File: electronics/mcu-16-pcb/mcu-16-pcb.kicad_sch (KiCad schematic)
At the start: 32 parts, among them J1 HRO_TYPE-C-31-M-12, J2 FFC Connector, U1 AP2112K-3.3, U2 W25Q64JVXGIQ, U3 Raspberry_Pi_RP2040, Y1 12MHz

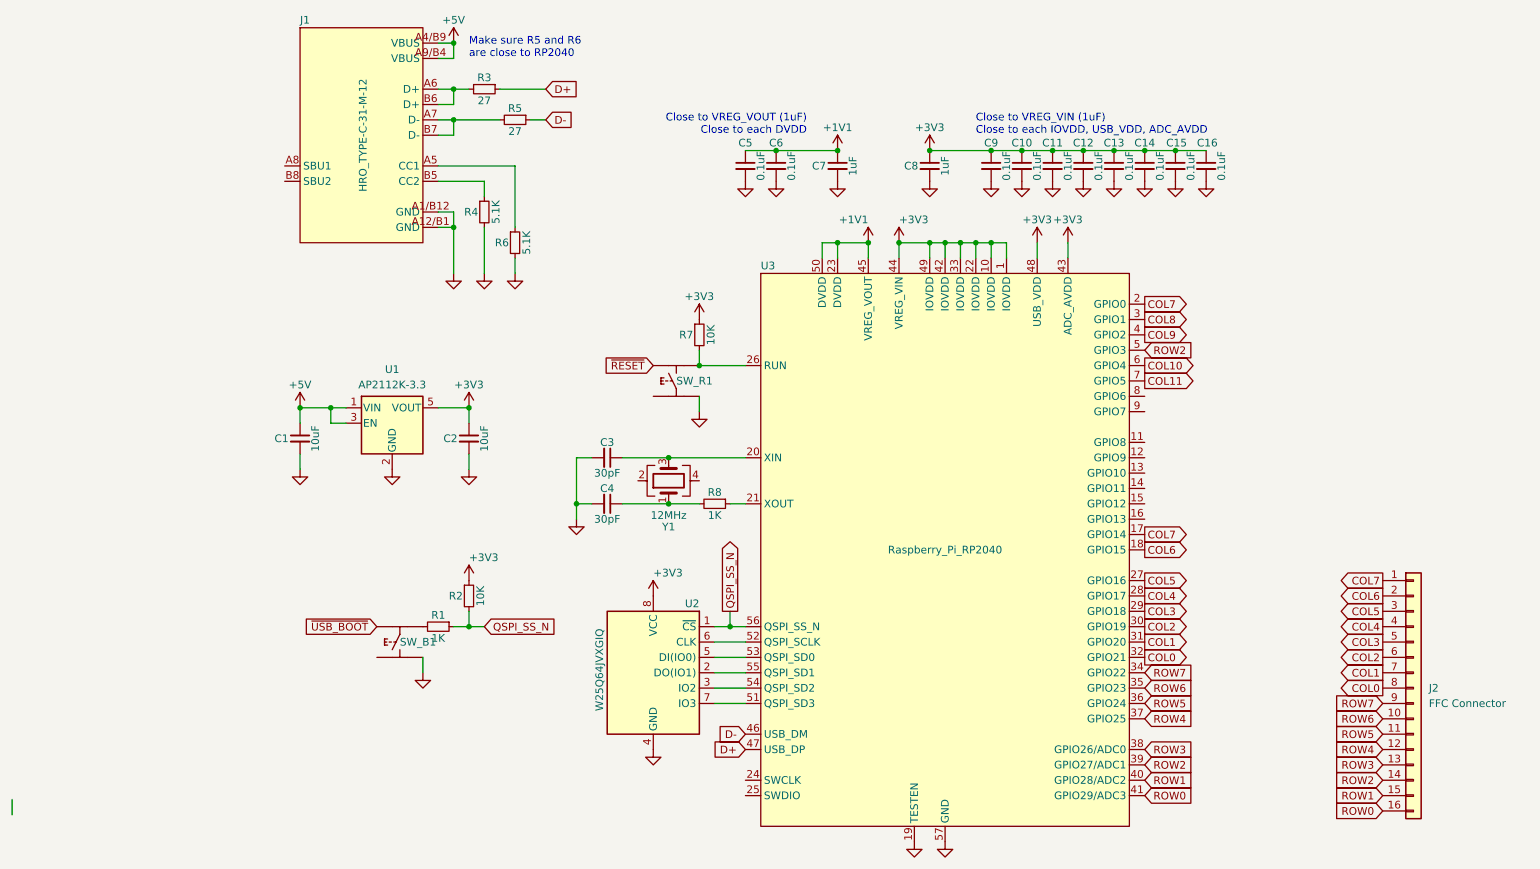
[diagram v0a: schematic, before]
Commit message: WIP Update
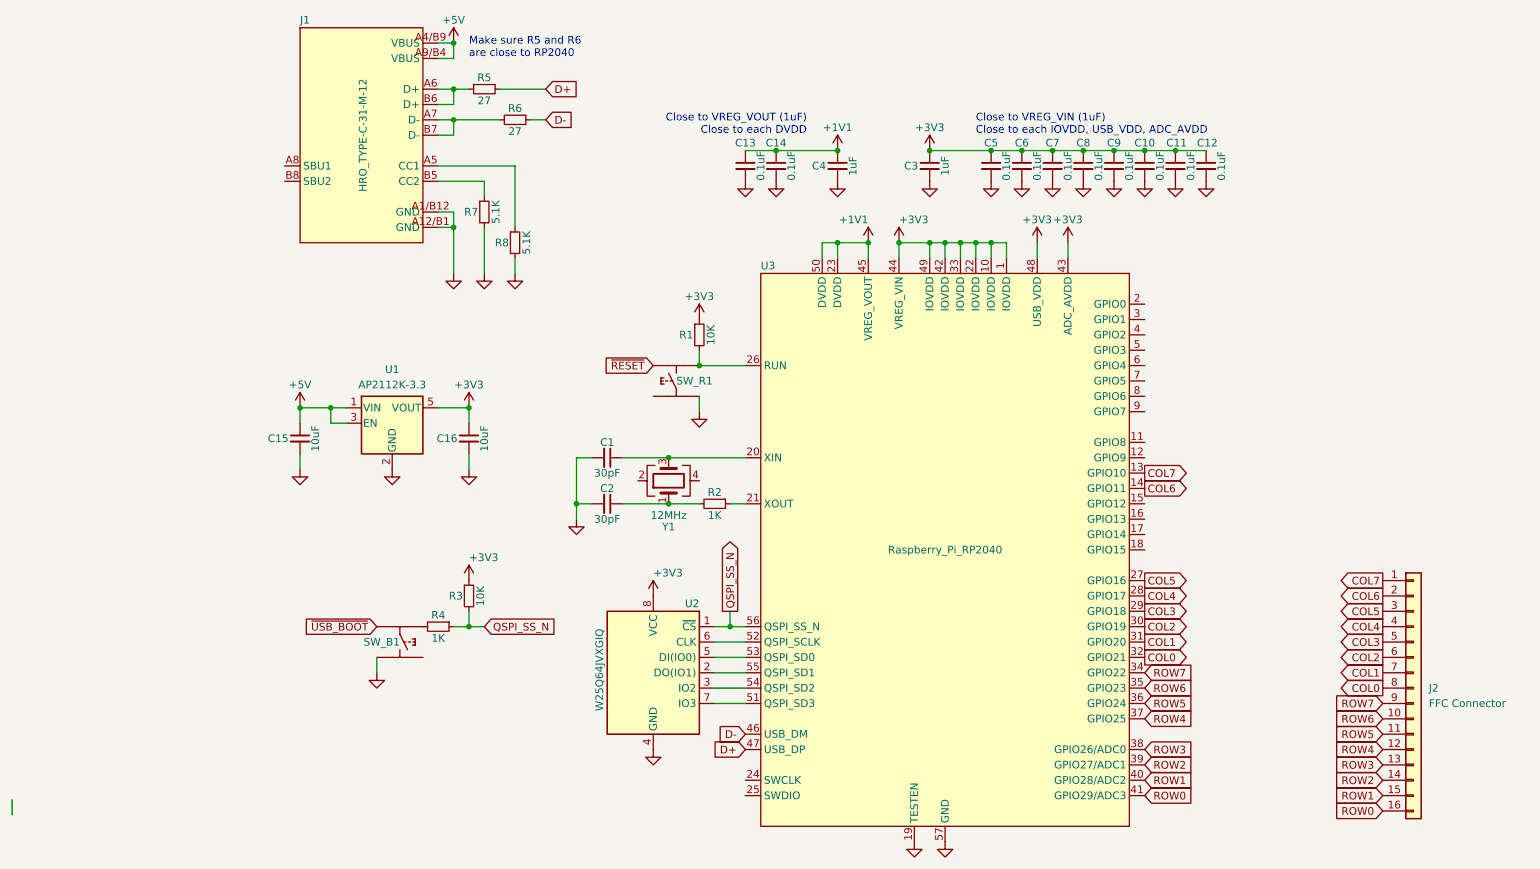
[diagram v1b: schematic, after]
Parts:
- renumbered C3 to C1, C14 to C10, C15 to C11, C16 to C12, C5 to C13, C6 to C14, C1 to C15, C2 to C16, C4 to C2, C8 to C3, C7 to C4, C9 to C5, C10 to C6, C11 to C7, C12 to C8, C13 to C9, R7 to R1, R8 to R2, R2 to R3, R1 to R4, R3 to R5, R5 to R6, R4 to R7, R6 to R8
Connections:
- net COL6: now also U3.14 (GPIO11); no longer U3.18 (GPIO15)
- net COL7: now also U3.13 (GPIO10); no longer U3.17 (GPIO14), U3.2 (GPIO0)
- net ROW2: no longer U3.5 (GPIO3)
- net ~{USB_BOOT}: now also SW_B1.1; no longer SW_B1.2
- net at R4.2: now also SW_B1.2; no longer SW_B1.1
- net COL10: no longer names the net of U3.6 (GPIO4)
- net COL11: no longer names the net of U3.7 (GPIO5)
- net COL8: no longer names the net of U3.3 (GPIO1)
- net COL9: no longer names the net of U3.4 (GPIO2)

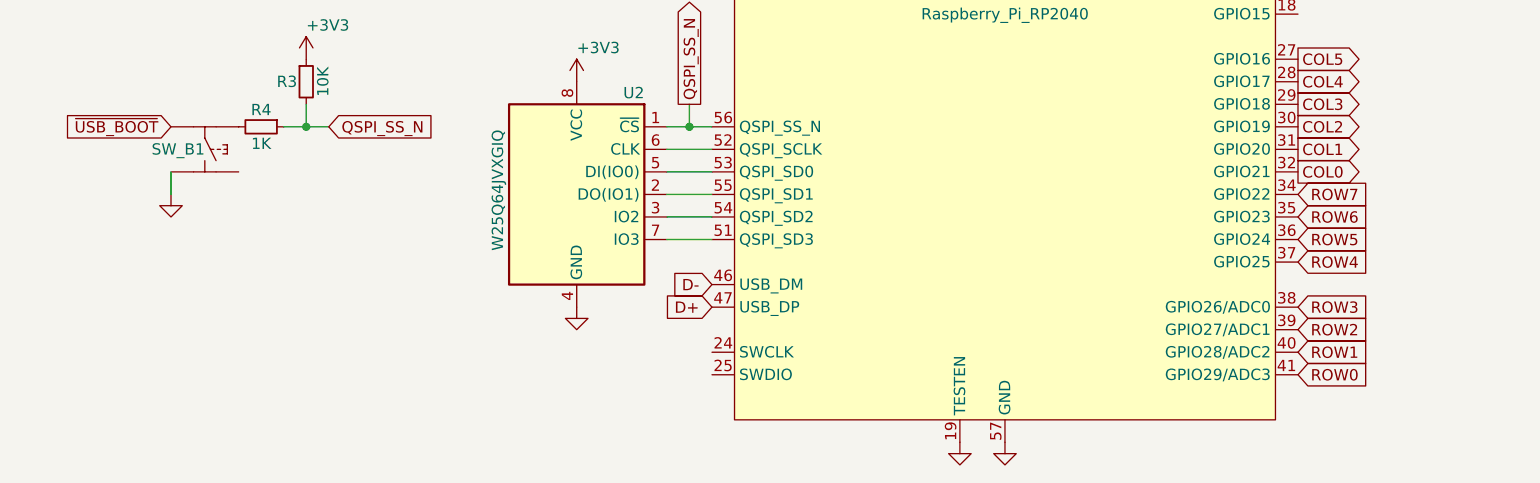
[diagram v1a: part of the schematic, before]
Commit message: Update MCU 16 pcb
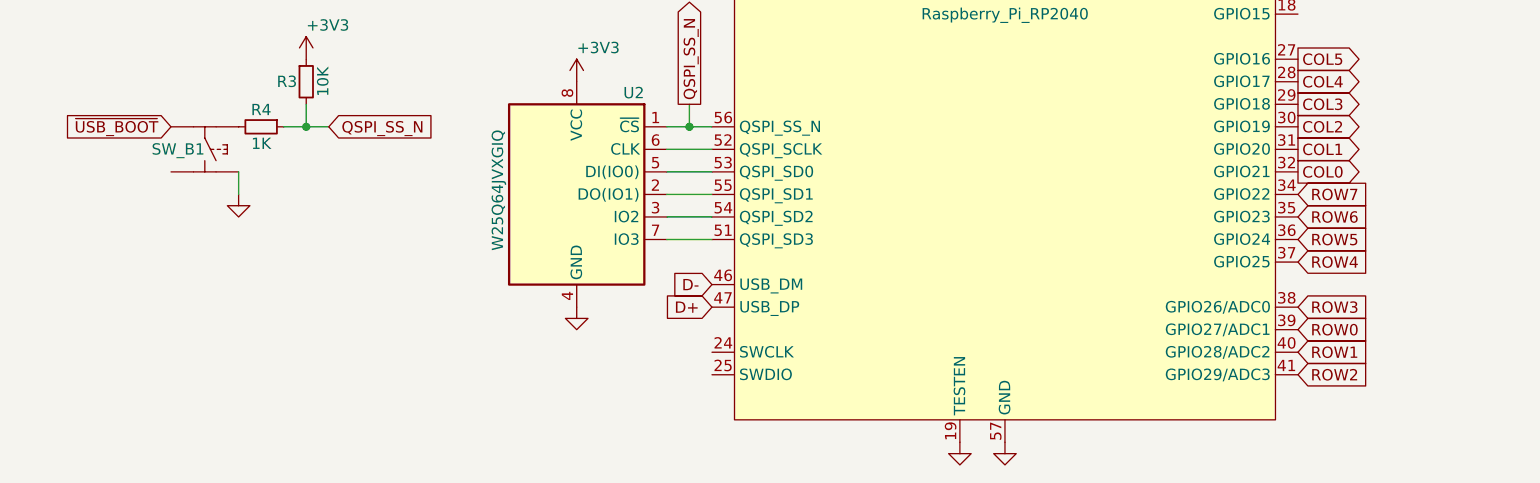
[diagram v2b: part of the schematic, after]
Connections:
- net GND: now also SW_B1.4; no longer SW_B1.3
- net ROW0: now also U3.39 (GPIO27/ADC1); no longer U3.41 (GPIO29/ADC3)
- net ROW2: now also U3.41 (GPIO29/ADC3); no longer U3.39 (GPIO27/ADC1)
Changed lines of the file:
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@@
 	(wire
 		(pts
-			(xy 35.56 127) (xy 35.56 129.54)
+			(xy 43.18 127) (xy 43.18 129.54)
 		)
 		(stroke
@@
 	(global_label "ROW2"
 		(shape input)
-		(at 162.56 144.78 0)
+		(at 162.56 149.86 0)
 		(fields_autoplaced yes)
 		(effects
@@
 		)
 		(property "Intersheetrefs" "${INTERSHEET_REFS}"
-			(at 170.8066 144.78 0)
+			(at 170.8066 149.86 0)
 			(effects
 				(font
@@
 	(global_label "ROW0"
 		(shape input)
-		(at 162.56 149.86 0)
+		(at 162.56 144.78 0)
 		(fields_autoplaced yes)
 		(effects
@@
 		)
 		(property "Intersheetrefs" "${INTERSHEET_REFS}"
-			(at 170.8066 149.86 0)
+			(at 170.8066 144.78 0)
 			(effects
 				(font
@@
 	(symbol
 		(lib_id "power:GND")
-		(at 35.56 129.54 0)
+		(at 43.18 129.54 0)
 		(unit 1)
 		(exclude_from_sim no)
@@
 		(fields_autoplaced yes)
 		(property "Reference" "#PWR04"
-			(at 35.56 135.89 0)
+			(at 43.18 135.89 0)
 			(effects
 				(font
@@
 		)
 		(property "Value" "GND"
-			(at 35.56 134.62 0)
+			(at 43.18 134.62 0)
 			(effects
 				(font
@@
 		)
 		(property "Footprint" ""
-			(at 35.56 129.54 0)
+			(at 43.18 129.54 0)
 			(effects
 				(font
@@
 		)
 		(property "Datasheet" ""
-			(at 35.56 129.54 0)
+			(at 43.18 129.54 0)
 			(effects
 				(font
@@
 		)
 		(property "Description" ""
-			(at 35.56 129.54 0)
-			(effects
-				(font
+			(at 43.18 129.54 0)
+			(effects
+				(font

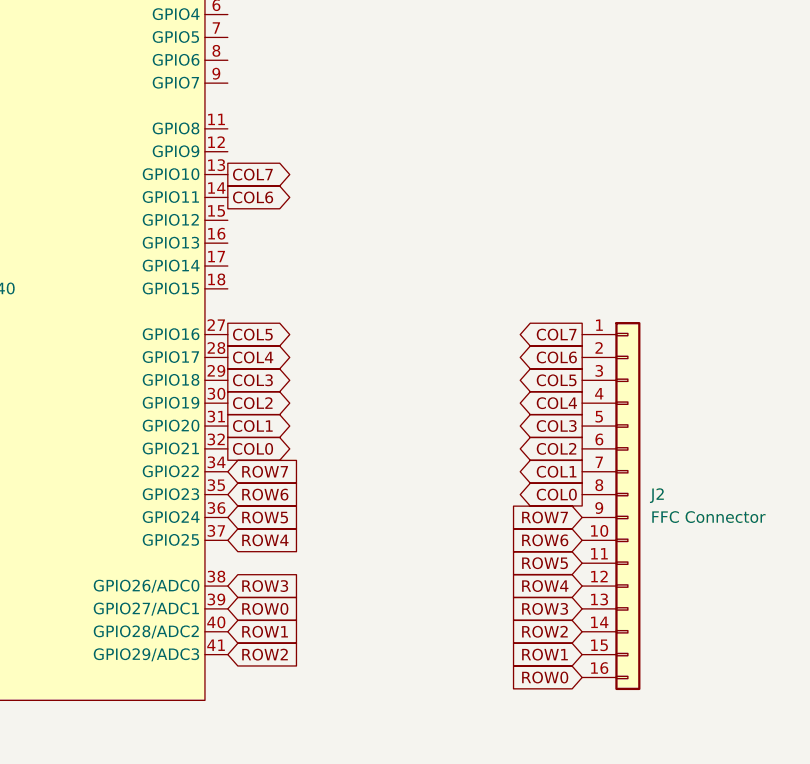
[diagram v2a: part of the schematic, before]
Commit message: Update MCU 16 pcb
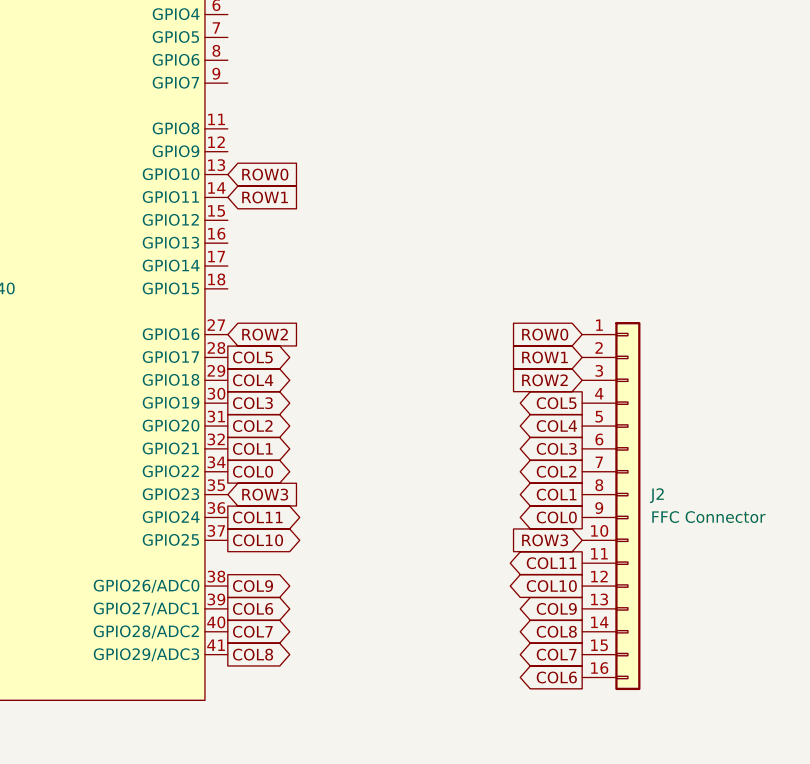
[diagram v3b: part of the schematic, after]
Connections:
- net ROW6 is gone; now on net ROW3: J2.10 (Pin_10), U3.35 (GPIO23)
- net ROW7 is gone; now on net COL0: J2.9 (Pin_9), U3.34 (GPIO22)
- net COL0: no longer J2.8 (Pin_8), U3.32 (GPIO21)
- net COL1: now also J2.8 (Pin_8), U3.32 (GPIO21); no longer J2.7 (Pin_7), U3.31 (GPIO20)
- net COL2: now also J2.7 (Pin_7), U3.31 (GPIO20); no longer J2.6 (Pin_6), U3.30 (GPIO19)
- net COL3: now also J2.6 (Pin_6), U3.30 (GPIO19); no longer J2.5 (Pin_5), U3.29 (GPIO18)
- net COL4: now also J2.5 (Pin_5), U3.29 (GPIO18); no longer J2.4 (Pin_4), U3.28 (GPIO17)
- net COL5: now also J2.4 (Pin_4), U3.28 (GPIO17); no longer J2.3 (Pin_3), U3.27 (GPIO16)
- net COL6: now also J2.16 (Pin_16), U3.39 (GPIO27/ADC1); no longer J2.2 (Pin_2), U3.14 (GPIO11)
- net COL7: now also J2.15 (Pin_15), U3.40 (GPIO28/ADC2); no longer J2.1 (Pin_1), U3.13 (GPIO10)
- net ROW0: now also J2.1 (Pin_1), U3.13 (GPIO10); no longer J2.16 (Pin_16), U3.39 (GPIO27/ADC1)
- net ROW1: now also J2.2 (Pin_2), U3.14 (GPIO11); no longer J2.15 (Pin_15), U3.40 (GPIO28/ADC2)
- net ROW2: now also J2.3 (Pin_3), U3.27 (GPIO16); no longer J2.14 (Pin_14), U3.41 (GPIO29/ADC3)
- net ROW3: no longer J2.13 (Pin_13), U3.38 (GPIO26/ADC0)
- net ROW4 renamed COL10
- net ROW5 renamed COL11
- new net COL8: J2.14 (Pin_14), U3.41 (GPIO29/ADC3)
- new net COL9: J2.13 (Pin_13), U3.38 (GPIO26/ADC0)

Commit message: Add MCU 16 files
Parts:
- SW_B1, SW_R1: LCSC C470426 -> C115360
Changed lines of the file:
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@@
 			)
 		)
-		(property "LCSC" "C470426"
+		(property "LCSC" "C115360"
 			(at 85.09 81.28 0)
 			(effects
@@
 			)
 		)
-		(property "LCSC" "C470426"
+		(property "LCSC" "C115360"
 			(at 39.37 124.46 0)
 			(effects
